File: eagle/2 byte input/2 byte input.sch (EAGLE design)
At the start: 26 parts, among them IC1 74LS165N, IC2 74LS165N, X3 MKDSN1,5/8-5,08, X5 MKDSN1,5/8-5,08

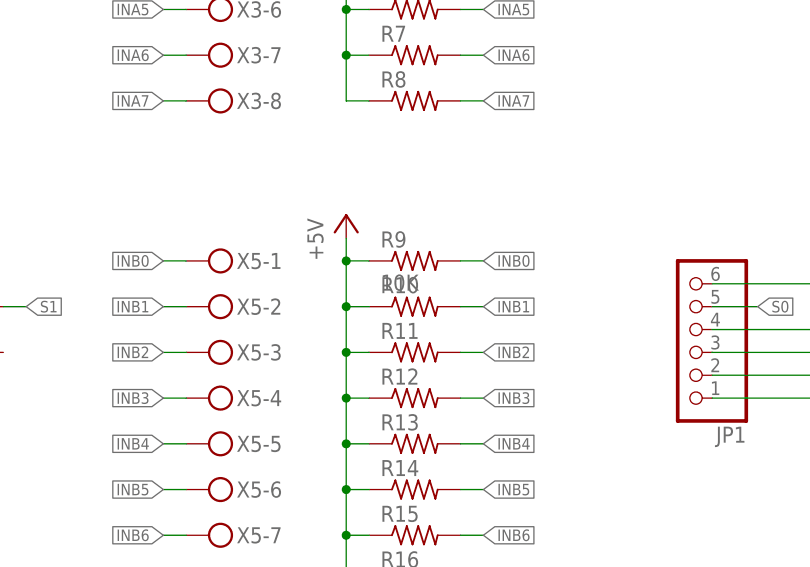
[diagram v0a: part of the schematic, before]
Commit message: periodic check-in
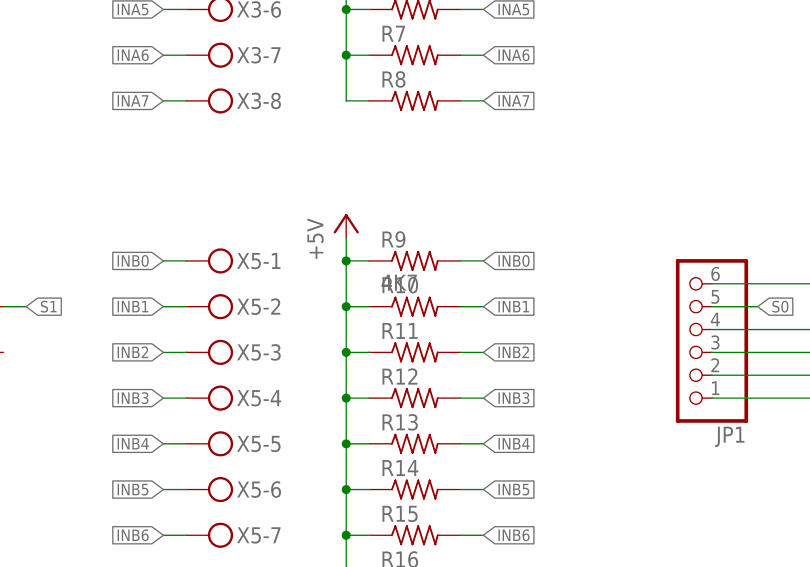
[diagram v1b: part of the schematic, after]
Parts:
- R9: value 10K -> 4K7
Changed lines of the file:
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@@
 <part name="R7" library="resistor" library_urn="urn:adsk.eagle:library:348" deviceset="R-US_" device="0207/2V" package3d_urn="urn:adsk.eagle:package:23490/1"/>
 <part name="R8" library="resistor" library_urn="urn:adsk.eagle:library:348" deviceset="R-US_" device="0207/2V" package3d_urn="urn:adsk.eagle:package:23490/1"/>
-<part name="R9" library="resistor" library_urn="urn:adsk.eagle:library:348" deviceset="R-US_" device="0207/2V" package3d_urn="urn:adsk.eagle:package:23490/1" value="10K"/>
+<part name="R9" library="resistor" library_urn="urn:adsk.eagle:library:348" deviceset="R-US_" device="0207/2V" package3d_urn="urn:adsk.eagle:package:23490/1" value="4K7"/>
 <part name="R10" library="resistor" library_urn="urn:adsk.eagle:library:348" deviceset="R-US_" device="0207/2V" package3d_urn="urn:adsk.eagle:package:23490/1"/>
 <part name="R11" library="resistor" library_urn="urn:adsk.eagle:library:348" deviceset="R-US_" device="0207/2V" package3d_urn="urn:adsk.eagle:package:23490/1"/>
